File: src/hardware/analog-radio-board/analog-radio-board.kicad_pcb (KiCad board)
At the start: 2 copper layers, 3 parts, among them J1 Conn_01x12_Male, J2 Conn_01x12_Male, U1 Si4735-D60-GU

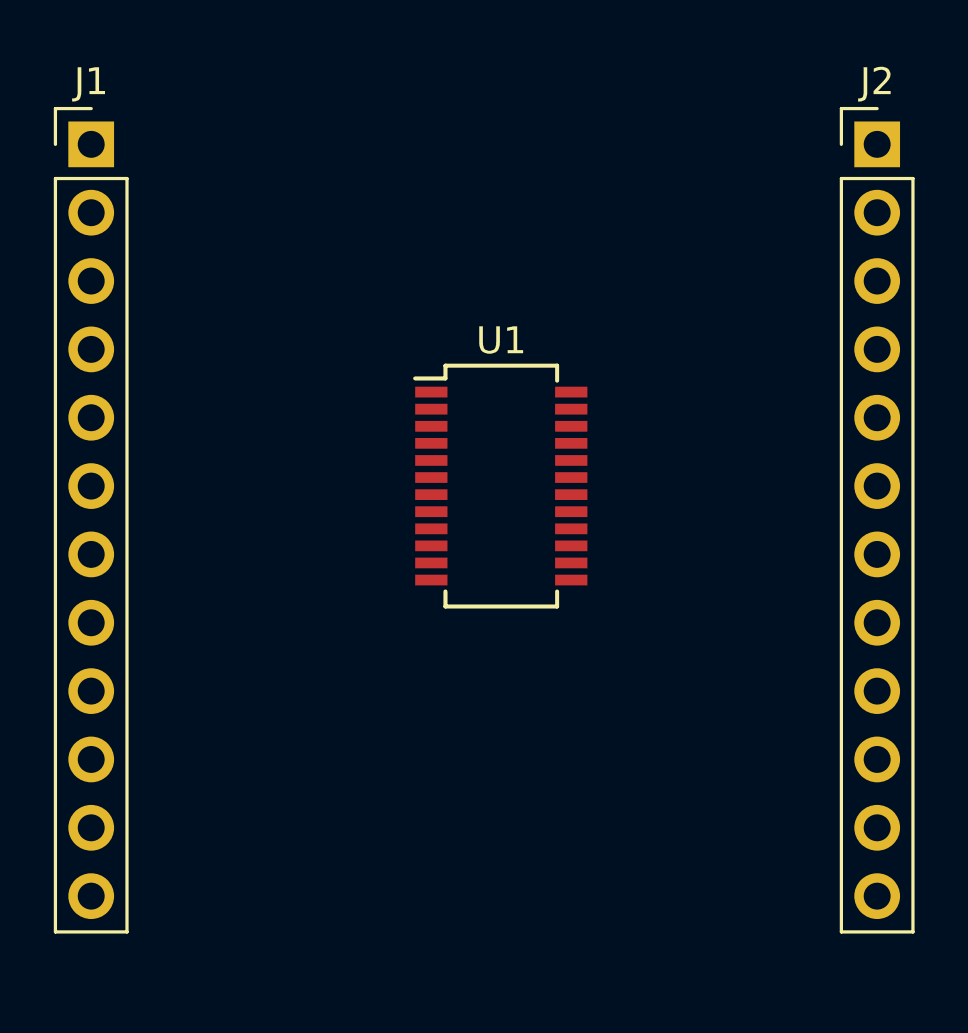
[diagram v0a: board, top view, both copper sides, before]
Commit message: feat: analog radio board v1.0.0
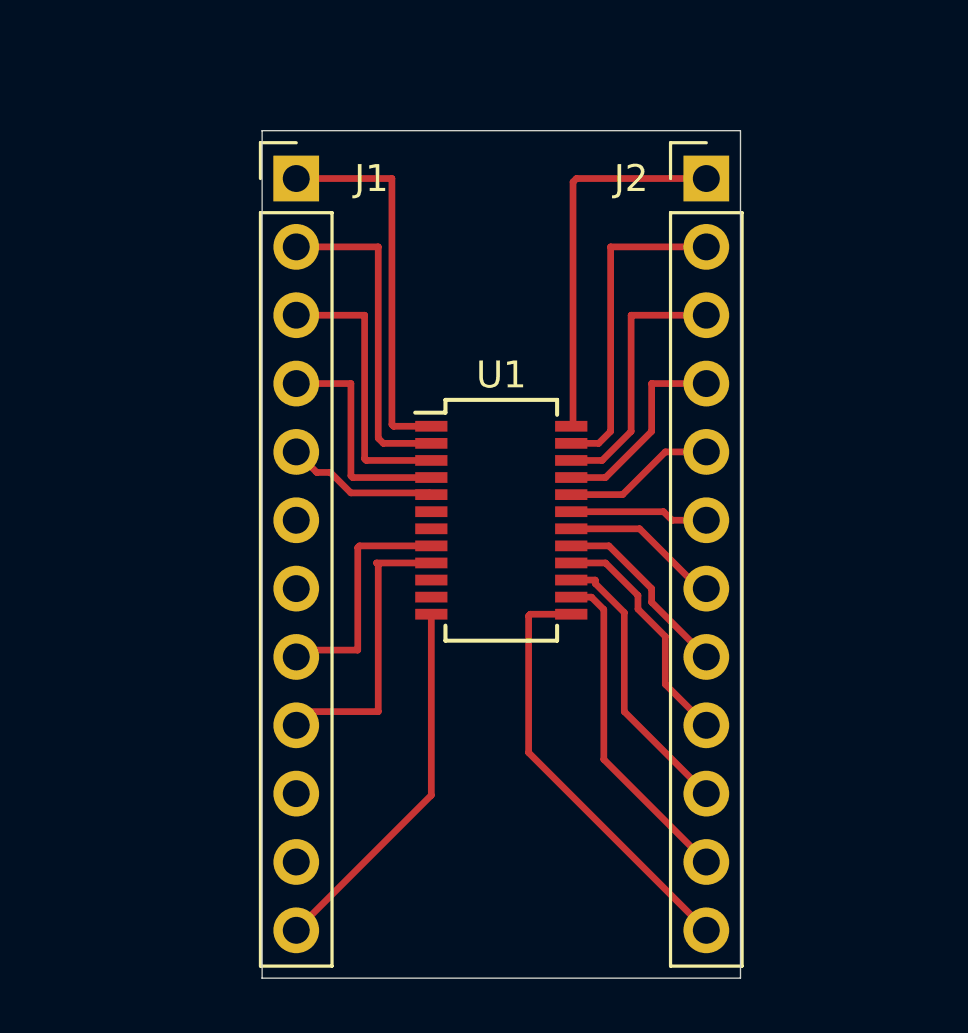
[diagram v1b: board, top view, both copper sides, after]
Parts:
- moved J1 7.73 mm to (133.3, 109.2)
- moved J2 6.48 mm to (148.6, 109.2)
- moved U1 1.27 mm to (141.0, 121.9)
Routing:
- net Net-(J2-Pad12): track 0.00 -> 16.0 mm
- net Net-(J1-Pad1): track 0.00 -> 14.3 mm
- net Net-(J2-Pad1): track 0.00 -> 14.1 mm
- net Net-(J1-Pad12): track 0.00 -> 13.8 mm
- net Net-(J2-Pad11): track 0.00 -> 12.4 mm
- net Net-(J1-Pad2): track 0.00 -> 12.2 mm
- net Net-(J2-Pad2): track 0.00 -> 12.1 mm
- net Net-(J1-Pad9): track 0.00 -> 10.8 mm
- net Net-(J2-Pad10): track 0.00 -> 10.5 mm
- net Net-(J1-Pad3): track 0.00 -> 10.4 mm
- net Net-(J2-Pad3): track 0.00 -> 9.79 mm
- net Net-(J1-Pad8): track 0.00 -> 8.96 mm
- net Net-(J2-Pad9): track 0.00 -> 8.86 mm
- net Net-(J1-Pad4): track 0.00 -> 8.48 mm
- net Net-(J2-Pad4): track 0.00 -> 7.51 mm
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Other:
- board outline added: 17.8 x 31.5 mm
- board text added: "oRadio anlog radio board v1.0.0 Designed in Berlin (c)2020"
